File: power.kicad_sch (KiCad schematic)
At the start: 28 parts, among them U5 TI LMR54410DBV, U7 TI LMR54410DBV

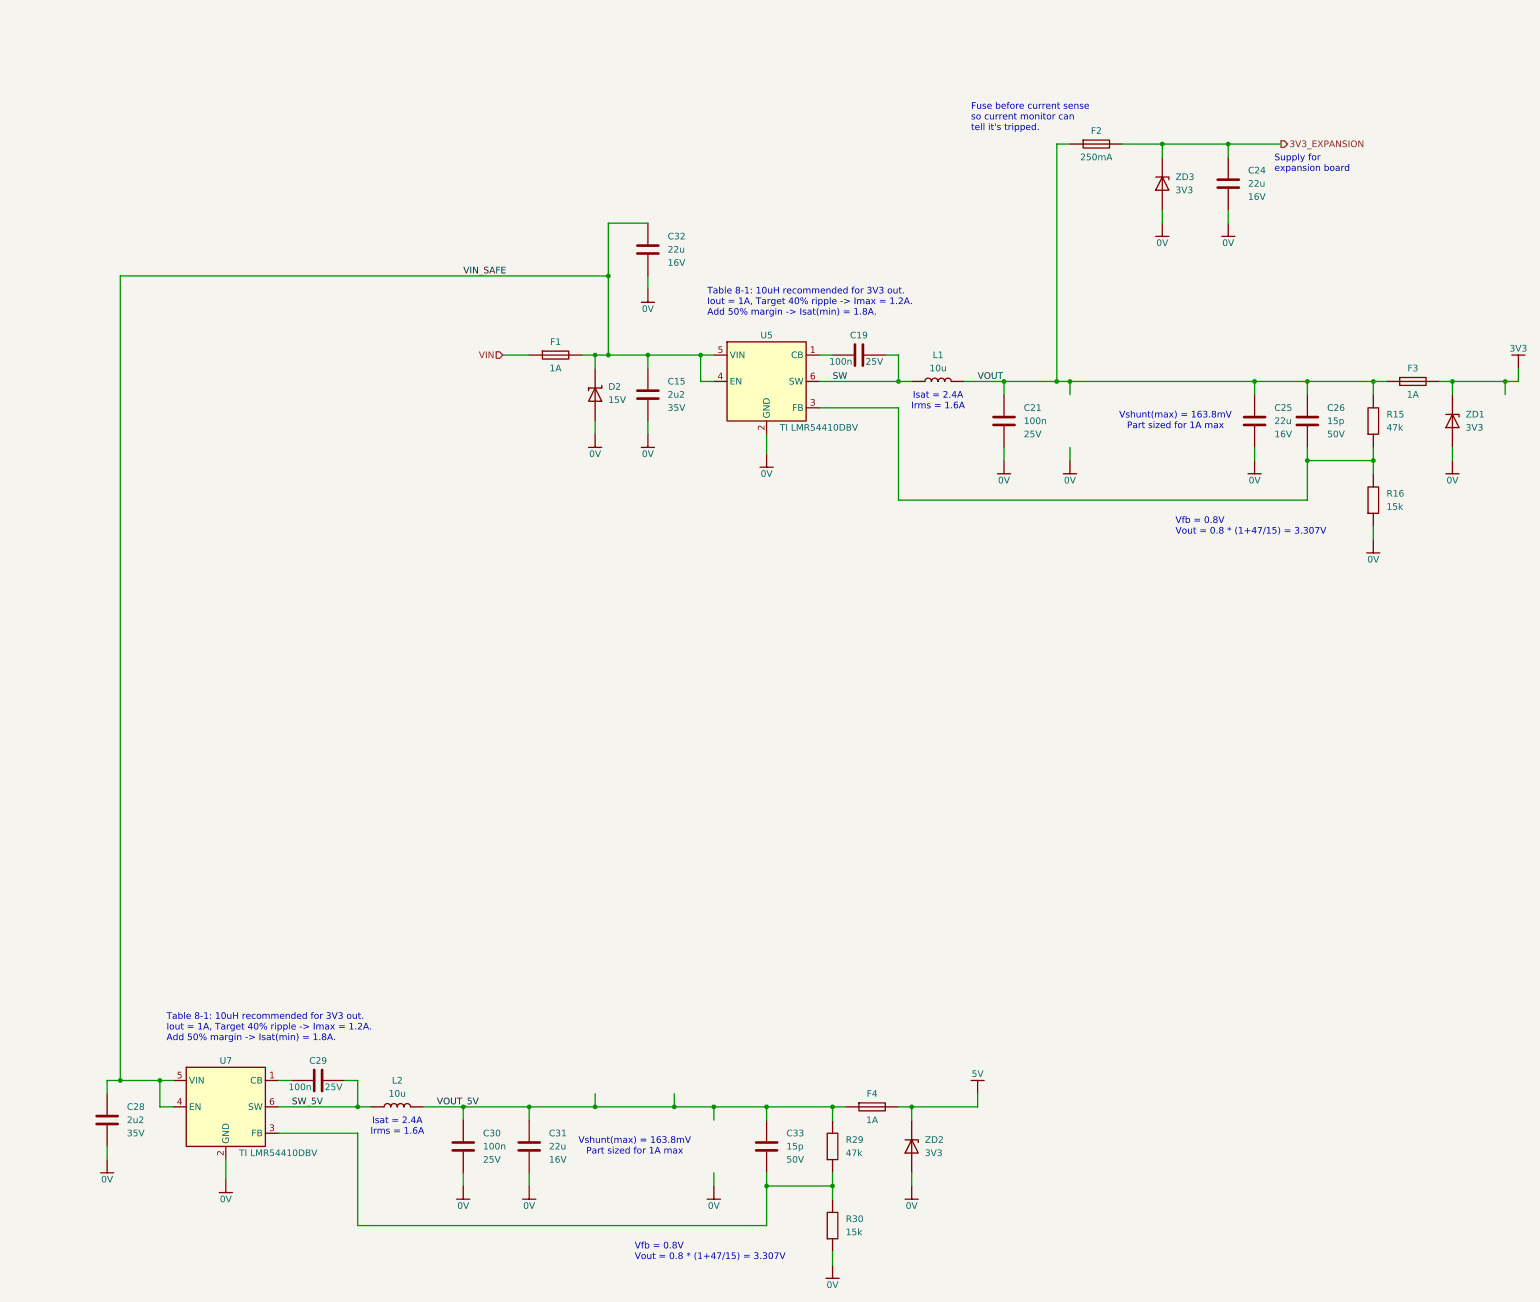
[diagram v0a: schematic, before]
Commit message: wup
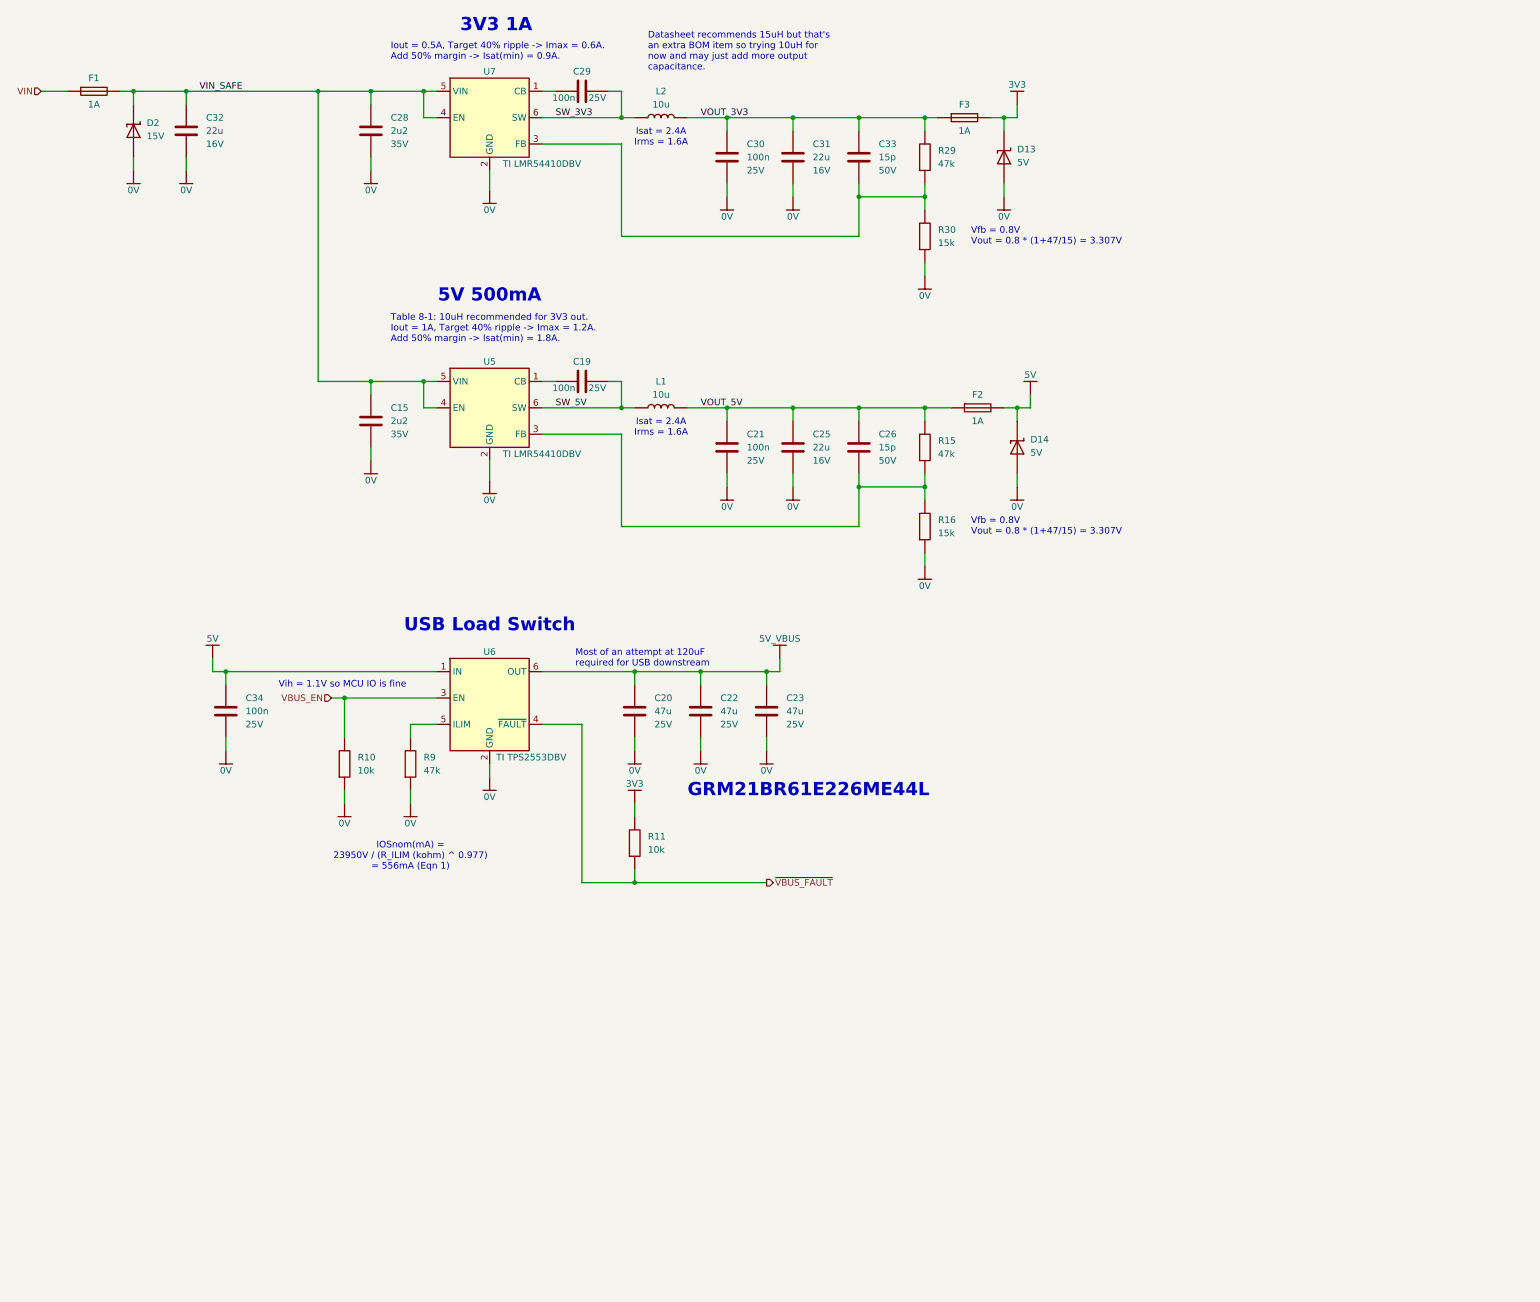
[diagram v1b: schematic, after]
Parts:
- removed C24: 22u, Capacitor_SMD:C_0603_1608Metric, symbol aaa_capacitor_auto_wut:Murata GRM188R61C226ME01
- removed F2: 250mA, Fuse:Fuse_0603_1608Metric, symbol fuse_auto_wut:Littelfuse 0603L025
- removed F4: 1A, Fuse:Fuse_0603_1608Metric, symbol fuse_auto_wut:Littelfuse 0467001.NR
- removed ZD1, ZD2, ZD3: 3V3, Diode_SMD:D_SOD-323, symbol tvs_zener_auto_wut:onsemi MM3Z3V3ST1G
- added C20, C22, C23: 47u, Capacitor_SMD:C_1206_3216Metric, symbol capacitor_auto_wut:TDK C3216X5R1E476M160AC
- added C34: 100n, Capacitor_WUT:C_0402_1005Metric, symbol aaa_capacitor_auto_wut:Yageo CC0402KRX7R8BB104
- added D13, D14: 5V, Diode_SMD:D_SOD-523, symbol aaa_tvs_zener_auto_wut:hongjiacheng H5VND5U
- added F2: 1A, Fuse:Fuse_0603_1608Metric, symbol fuse_auto_wut:Littelfuse 0467001.NR
- added R10, R11: 10k, Resistor_WUT:R_0402_1005Metric, symbol aaa_resistor_auto_wut:KOA Speer RK73H1ETTP1002F
- added R9: 47k, Resistor_WUT:R_0402_1005Metric, symbol resistor_auto_wut:KOA Speer RK73H1ETTP4702F
- added U6: TI TPS2553DBV, IC_WUT:SOT-23-6, symbol IC_WUT:TPS2553DBV
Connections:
- net SW is gone; now on net SW_5V: C19.1, L1.1, U5.6 (SW)
- net 0V: now also C20.2, C22.2, C23.2, C34.2, D13.2 (A), D14.2 (A), R10.2, R9.2, U6.2 (GND)
- net 3V3: now also D13.1 (K), R11.1
- net 5V: now also C34.1, D14.1 (K), F2.2, U6.1 (IN)
- net SW_5V: no longer C29.1, L2.1, U7.6 (SW)
- net VOUT_5V: now also C21.1, C25.1, C26.1, L1.2, R15.1, F2.1; no longer C30.1, C31.1, C33.1, L2.2, R29.1
- removed net VOUT: C21.1, C25.1, C26.1, F3.1, L1.2, R15.1
- new net: R9.1, U6.5 (ILIM)
- new net 5V_VBUS: C20.1, C22.1, C23.1, U6.6 (OUT)
- new net SW_3V3: C29.1, L2.1, U7.6 (SW)
- new net VBUS_EN: R10.1, U6.3 (EN)
- new net VOUT_3V3: C30.1, C31.1, C33.1, F3.1, L2.2, R29.1
- new net ~{VBUS_FAULT}: R11.2, U6.4 (~{FAULT})
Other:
- note added: "3V3 1A"
- note added: "5V 500mA"
- note added: "Datasheet recommends 15uH but that's an extra BOM item so trying 10uH for now and may just add more output capacitance."
- note added: "GRM21BR61E226ME44L"
- note added: "IOSnom(mA) = 23950V / (R_ILIM (kohm) ^ 0.977) = 556mA (Eqn 1)"
- note added: "Iout = 0.5A, Target 40% ripple -> Imax = 0.6A. Add 50% margin -> Isat(min) = 0.9A."
- note added: "Most of an attempt at 120uF required for USB downstream"
- note added: "USB Load Switch"
- note added: "Vih = 1.1V so MCU IO is fine"
- note removed: "Fuse before current sense so current monitor can tell it's tripped."
- note removed: "Supply for expansion board"
- note removed: "Vshunt(max) = 163.8mV Part sized for 1A max"
- moved on the sheet: C15, C19, C21, C25, C26, C28, C29, C30, C31, C33, D2, F1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
